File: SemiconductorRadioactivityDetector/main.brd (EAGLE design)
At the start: 32 parts, among them IC1 317T, IC3 LM324N, Q1 2N4093

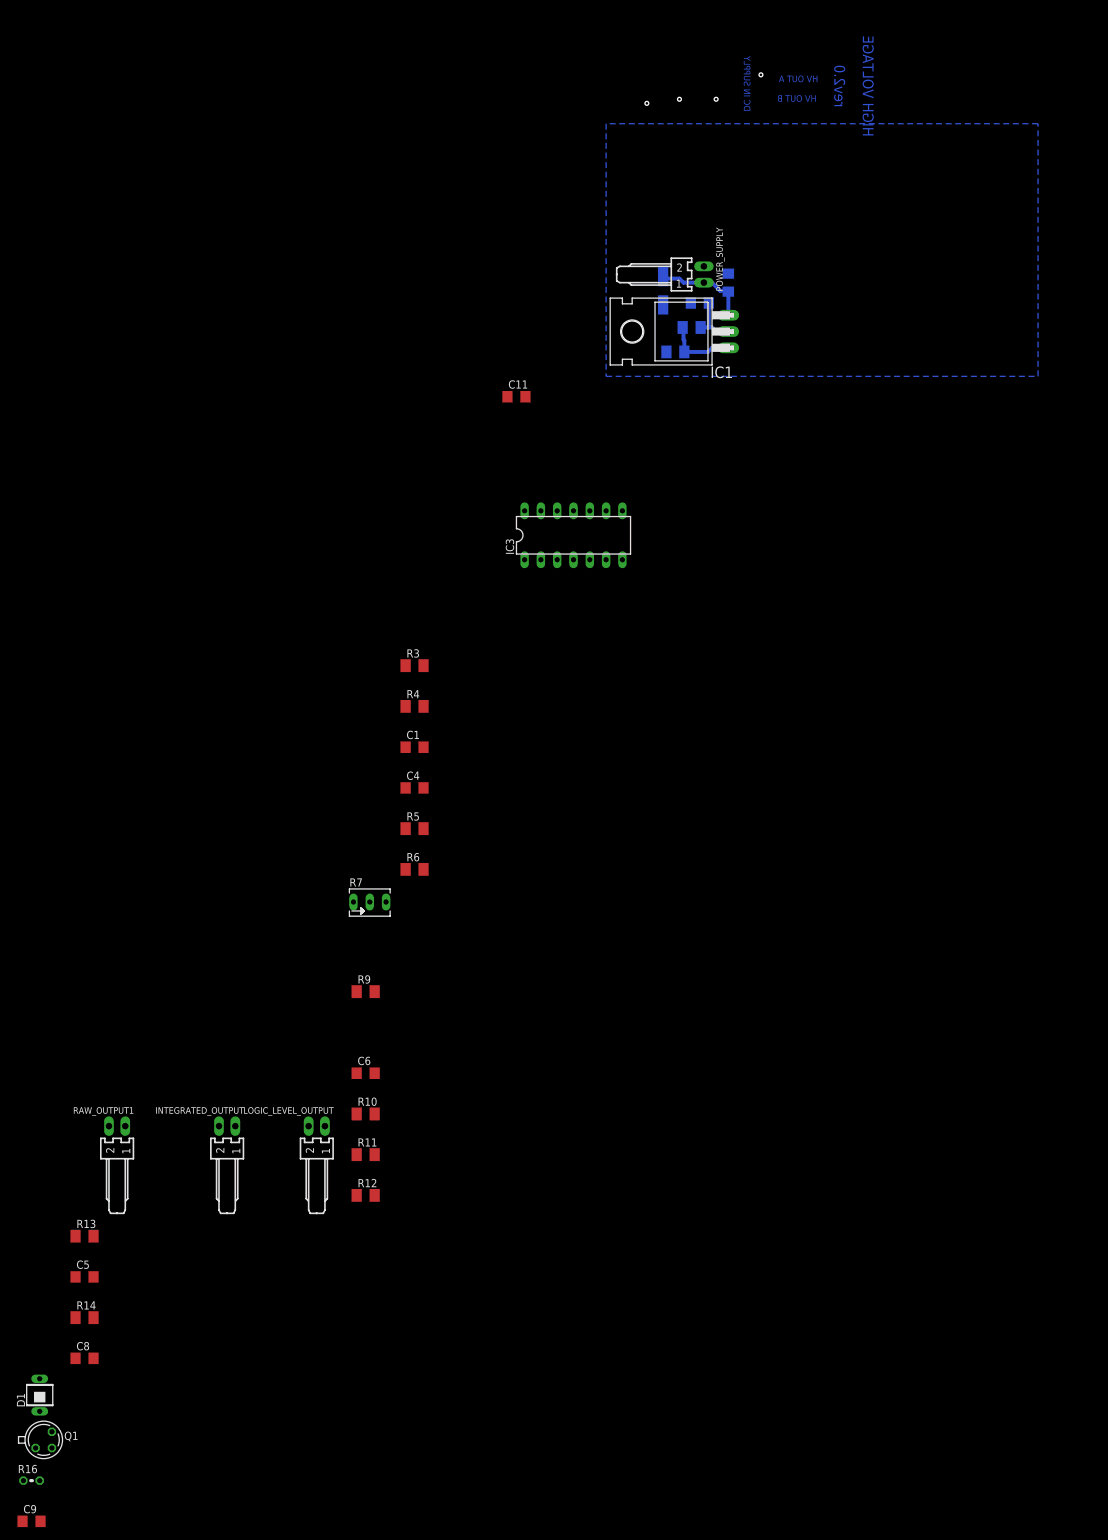
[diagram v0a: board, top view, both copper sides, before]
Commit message: PCB done.
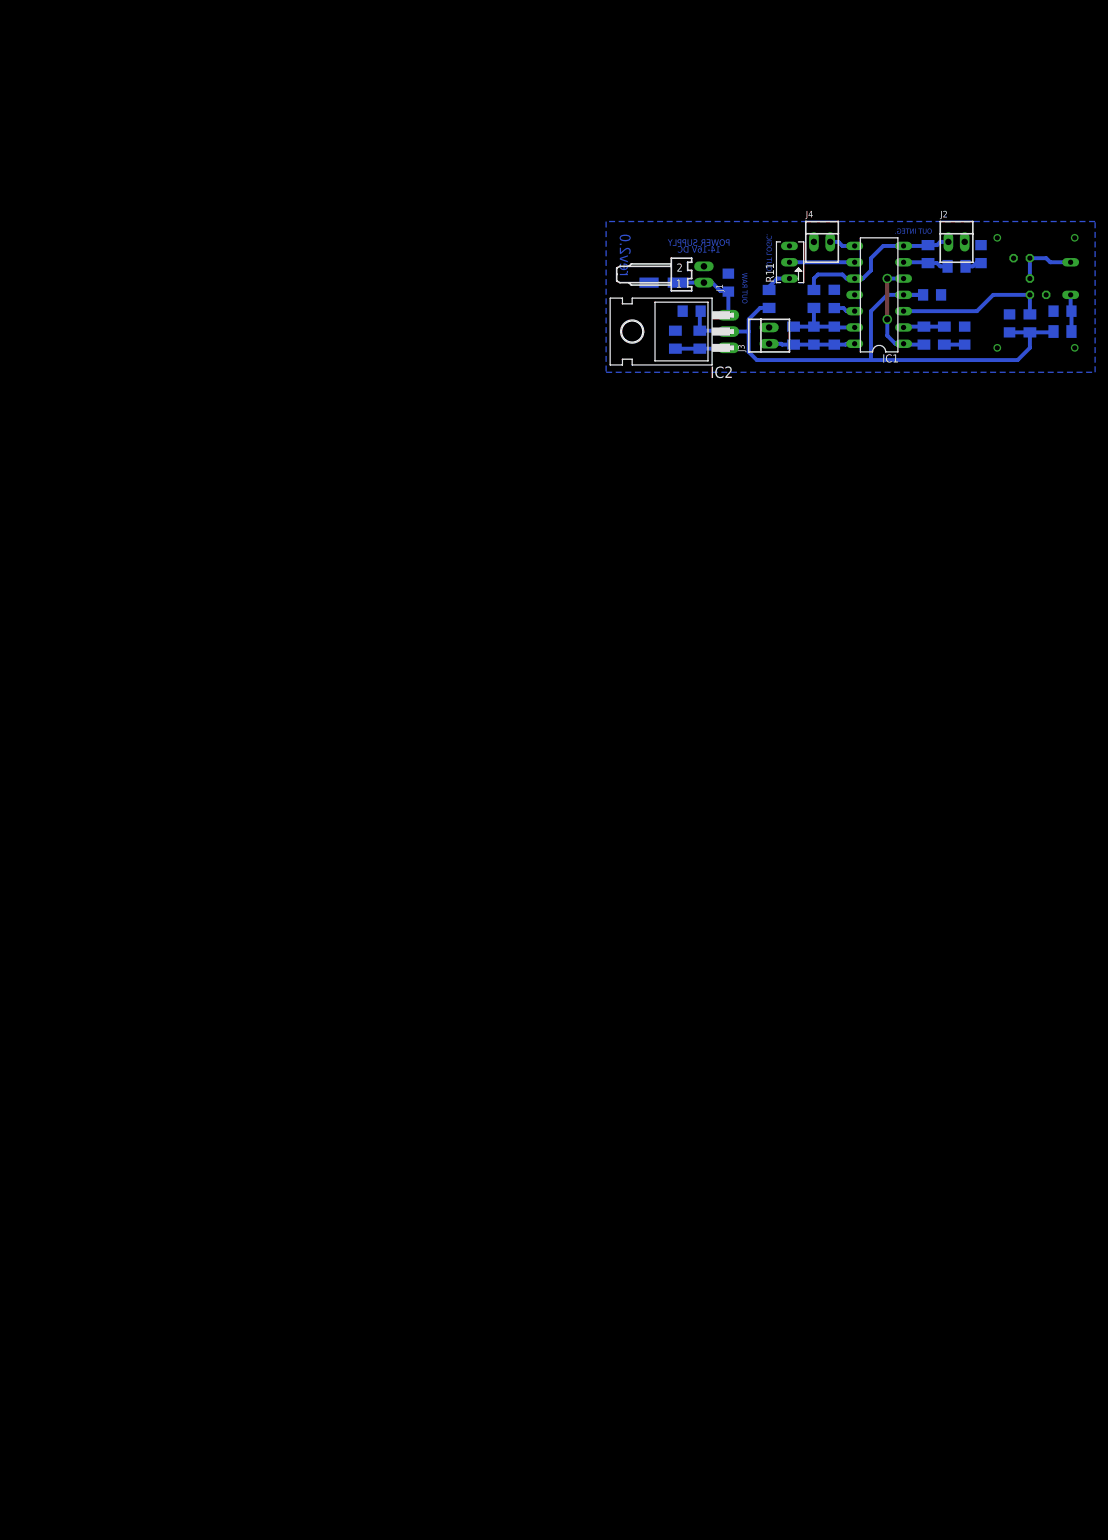
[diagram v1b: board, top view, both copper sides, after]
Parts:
- removed C11: 100n, resistor:C1206
- removed IC3: LM324N, linear:DIL14
- removed INTEGRATED_OUTPUT, LOGIC_LEVEL_OUTPUT, RAW_OUTPUT1: 22-05-7028-02, con-molex:7395-02
- removed R16: 10M, resistor:0204V
- added C10: 100n, resistor:C1206
- added IC2: 317T, linear:TO220H
- added J2, J3, J4: 22-23-2021, con-molex:22-23-2021
- added R8: 240R, resistor:M1206
- C1: value 15n -> 100n
- C6: value 100n -> 15n
- IC1: value 317T -> LM324N; device linear:TO220H -> linear:DIL14
- R1: value 240R -> 10M; device resistor:M1206 -> resistor:0204V
- R10: value 1M -> 4k7
- R11: value 100k -> 1k; device resistor:M1206 -> pot:B64Y
- R12: device resistor:M1206 -> resistor:R1206
- R13: value 1M -> 100k
- R14: value 47k -> 1M
- R2: value 2k -> 1M
- R3: value 1M -> 47k
- R5: value 100k -> 1M
- R7: value 1k -> 100k; device pot:B64Y -> resistor:M1206
- R9: value 4k7 -> 2k
- moved Q1 237.3 mm to (67.3, 14.0), flipped to the bottom
- moved D1 236.8 mm to (72.4, 15.2), flipped to the bottom
- moved C9 221.4 mm to (32.4, 6.35), flipped to the bottom, turned to 270 degrees
- moved R14 188.8 mm to (29.2, 6.35), flipped to the bottom, turned to 90 degrees
- moved C8 188.6 mm to (13.3, 10.2), flipped to the bottom
- moved R13 185.1 mm to (32.4, 12.1), flipped to the bottom, turned to 90 degrees
- moved C5 184.6 mm to (19.1, 14.6), flipped to the bottom, turned to 90 degrees
- moved C6 159.6 mm to (58.4, 19.1), flipped to the bottom, turned to 90 degrees
- moved R12 157.6 mm to (35.6, 12.1), flipped to the bottom, turned to 270 degrees
- moved R11 153.9 mm to (28.6, 17.8), turned to 90 degrees
- moved R10 141.7 mm to (25.4, 12.1), flipped to the bottom, turned to 90 degrees
- moved R7 133.3 mm to (50.2, 19.1), flipped to the bottom, turned to 270 degrees
- moved R6 126.4 mm to (54.6, 17.1), flipped to the bottom
- moved C1 121.7 mm to (71.1, 10.2), flipped to the bottom
- moved R9 112.5 mm to (10.8, 5.71), flipped to the bottom, turned to 270 degrees
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- renumbered POWER_SUPPLY to J1
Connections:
- net GND: now also C6.2, IC1.11, J2.2, J3.2, J4.1, R1.2, R11.A, R9.1; no longer C11.2, IC3.11, INTEGRATED_OUTPUT.2, LOGIC_LEVEL_OUTPUT.1, R16.2, R2.1, R7.A, RAW_OUTPUT1.2
- net N$1: now also IC2.1, R8.1, R9.2; no longer IC1.1, R1.1, R2.2
- net N$11: now also IC1.9, R11.S; no longer IC3.9, R7.S
- net N$12: now also C10.1, IC1.13, R13.1, R14.2; no longer C6.1, IC3.13, R10.2, R11.1
- net N$13: now also C10.2, IC1.14, J3.1, R14.1; no longer C6.2, IC3.14, INTEGRATED_OUTPUT.1, R10.1
- net N$14: now also IC1.12; no longer IC3.12
- net N$15: now also IC1.8, J4.2; no longer IC3.8, LOGIC_LEVEL_OUTPUT.2
- net N$16: now also C1.1, R2.2; no longer C5.1, R13.2
- net N$17: now also R1.1; no longer R16.1
- net N$18: now also IC1.3, R3.1; no longer IC3.3, R14.1
- net N$19: now also IC1.10, IC1.7, J2.1, R13.2, R7.1; no longer IC3.10, IC3.7, R11.2, R5.1, RAW_OUTPUT1.1
- net N$2: now also IC1.2, R5.2; no longer IC3.2, R3.2
- net N$3: now also IC1.1, IC1.5, R5.1; no longer IC3.1, IC3.5, R3.1
- net N$4: now also C4.1; no longer C1.1
- net N$5: now also IC1.6, R7.2; no longer IC3.6, R5.2
- net N$7: now also C6.1; no longer C4.1
- net N$8: now also C5.1, IC2.3; no longer C2.1, IC1.3
- net N$9: now also R10.2, R11.E; no longer R7.E, R9.2
- net VCC: now also C2.1, IC1.4, IC2.2, R10.1, R2.1, R3.2, R8.2; no longer C11.1, IC1.2, IC3.4, R1.2, R13.1, R14.2, R9.1
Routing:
- net VCC: track 8.44 -> 94.1 mm
- net N$19: track 0.00 -> 26.7 mm
- net N$18: track 0.00 -> 23.8 mm
- net N$3: track 0.00 -> 17.7 mm, vias 0 -> 2
- net N$13: track 0.00 -> 13.4 mm
- net N$12: track 0.00 -> 12.5 mm
- net N$11: track 0.00 -> 10.2 mm
- net N$17: track 0.00 -> 9.79 mm
- net N$5: track 0.00 -> 7.12 mm
- net N$2: track 0.00 -> 6.40 mm
- net N$16: track 0.00 -> 5.77 mm
- net N$9: track 0.00 -> 4.21 mm
- net N$15: track 0.00 -> 4.07 mm
- net N$14: track 0.00 -> 3.38 mm
- net N$4: track 0.00 -> 3.18 mm
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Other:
- board text added: "OUT INTEG."
- board text added: "OUT LOGIC."
- board text added: "OUT RAW"
- board text added: "POWER SUPPLY 14-16V DC"
- board text removed: "DC IN SUPPLY"
- board text removed: "HIGH VOLTAGE"
- board text removed: "HV OUT A"
- board text removed: "HV OUT B"
